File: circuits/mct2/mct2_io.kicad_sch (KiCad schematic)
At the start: 72 parts

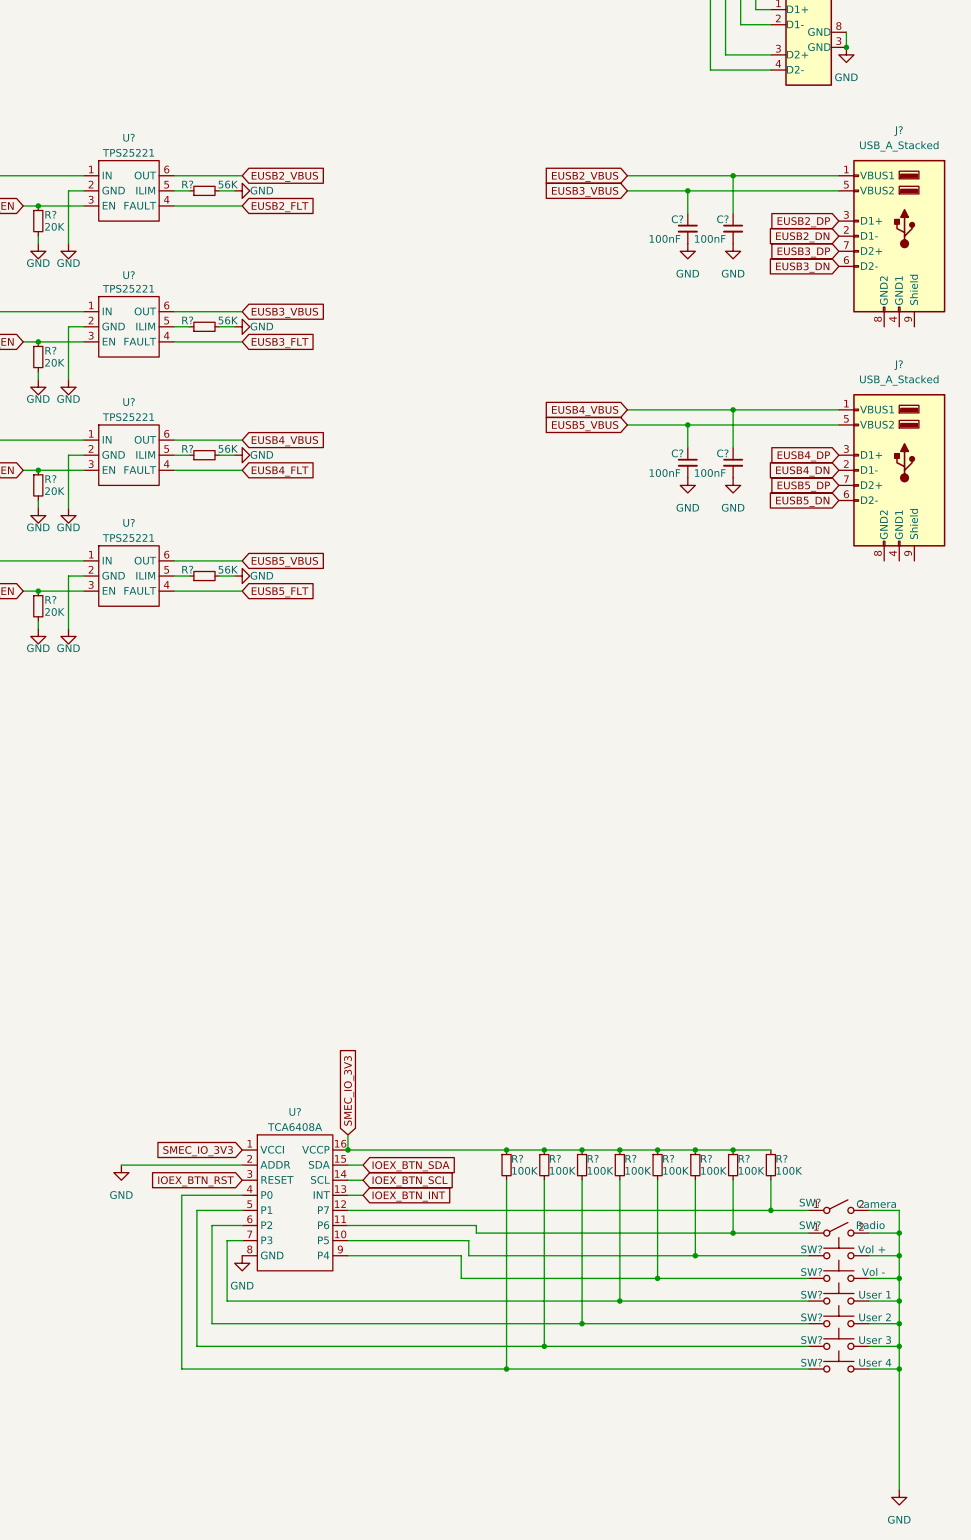
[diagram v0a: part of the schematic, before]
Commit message: July 27, 2024
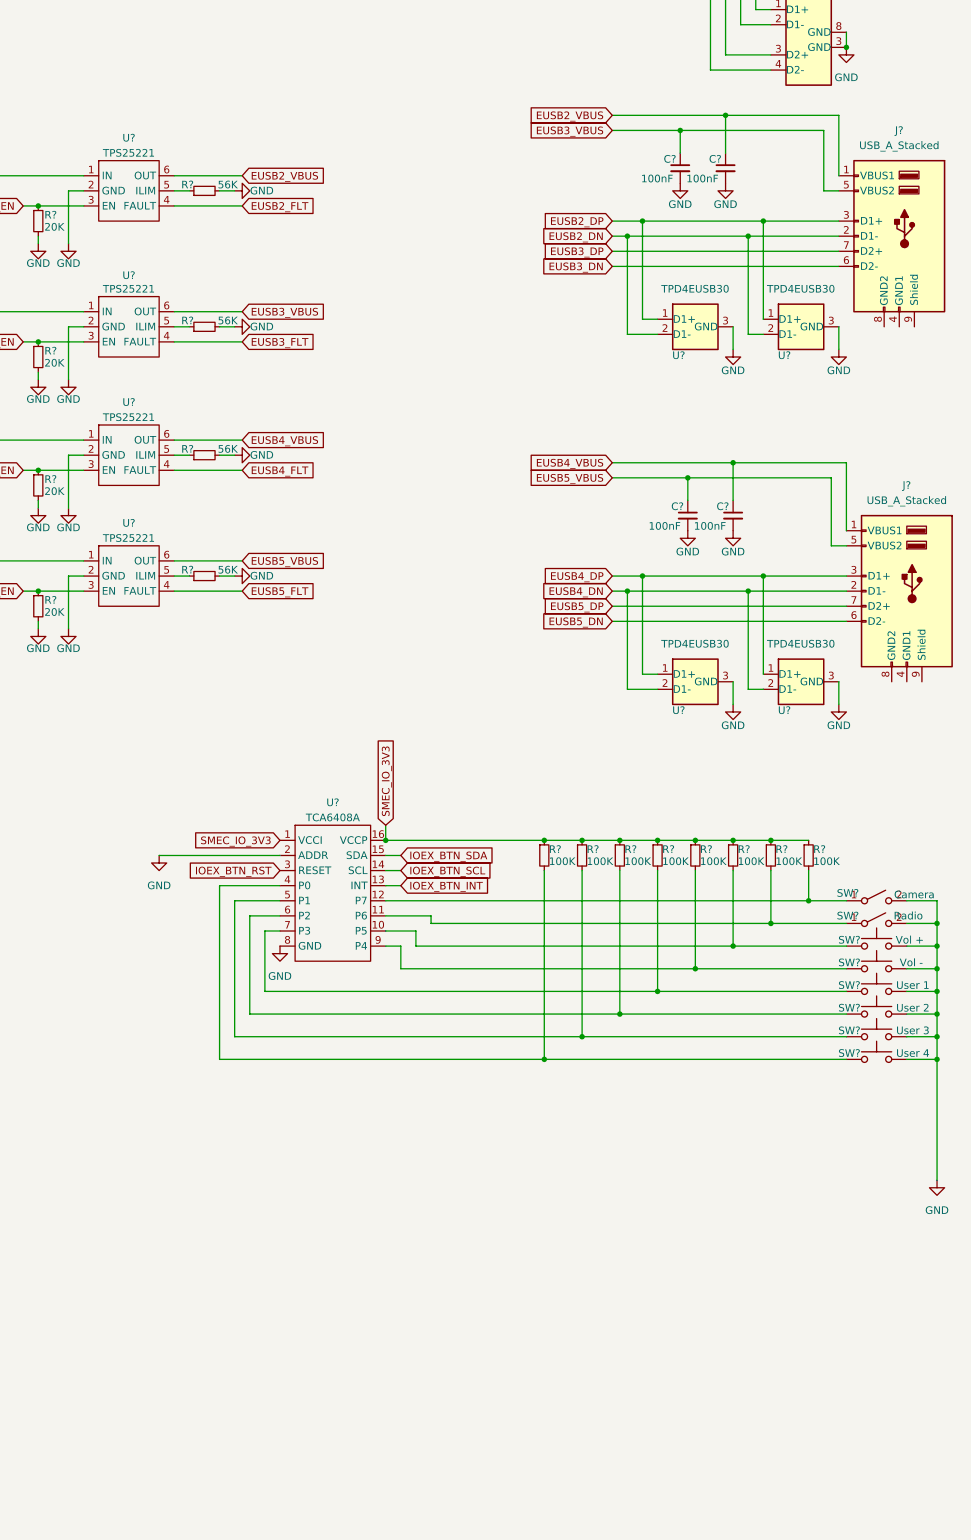
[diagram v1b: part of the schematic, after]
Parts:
- added U? (x4): TPD4EUSB30, Package_TO_SOT_SMD:Texas_DRT-3, symbol mediacow:TPD2EUSB30
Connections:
- net EUSB2_DN: now also U?.2 (D1-), U?.2 (D1-)
- net EUSB2_DP: now also U?.1 (D1+), U?.1 (D1+)
- net EUSB4_DN: now also U?.2 (D1-), U?.2 (D1-)
- net EUSB4_DP: now also U?.1 (D1+), U?.1 (D1+)
- net GND: now also U?.3 (GND), U?.3 (GND), U?.3 (GND), U?.3 (GND)
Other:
- moved on the sheet: C?, J?, R?, SW?, U?
